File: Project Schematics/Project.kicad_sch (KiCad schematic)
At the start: 9 parts

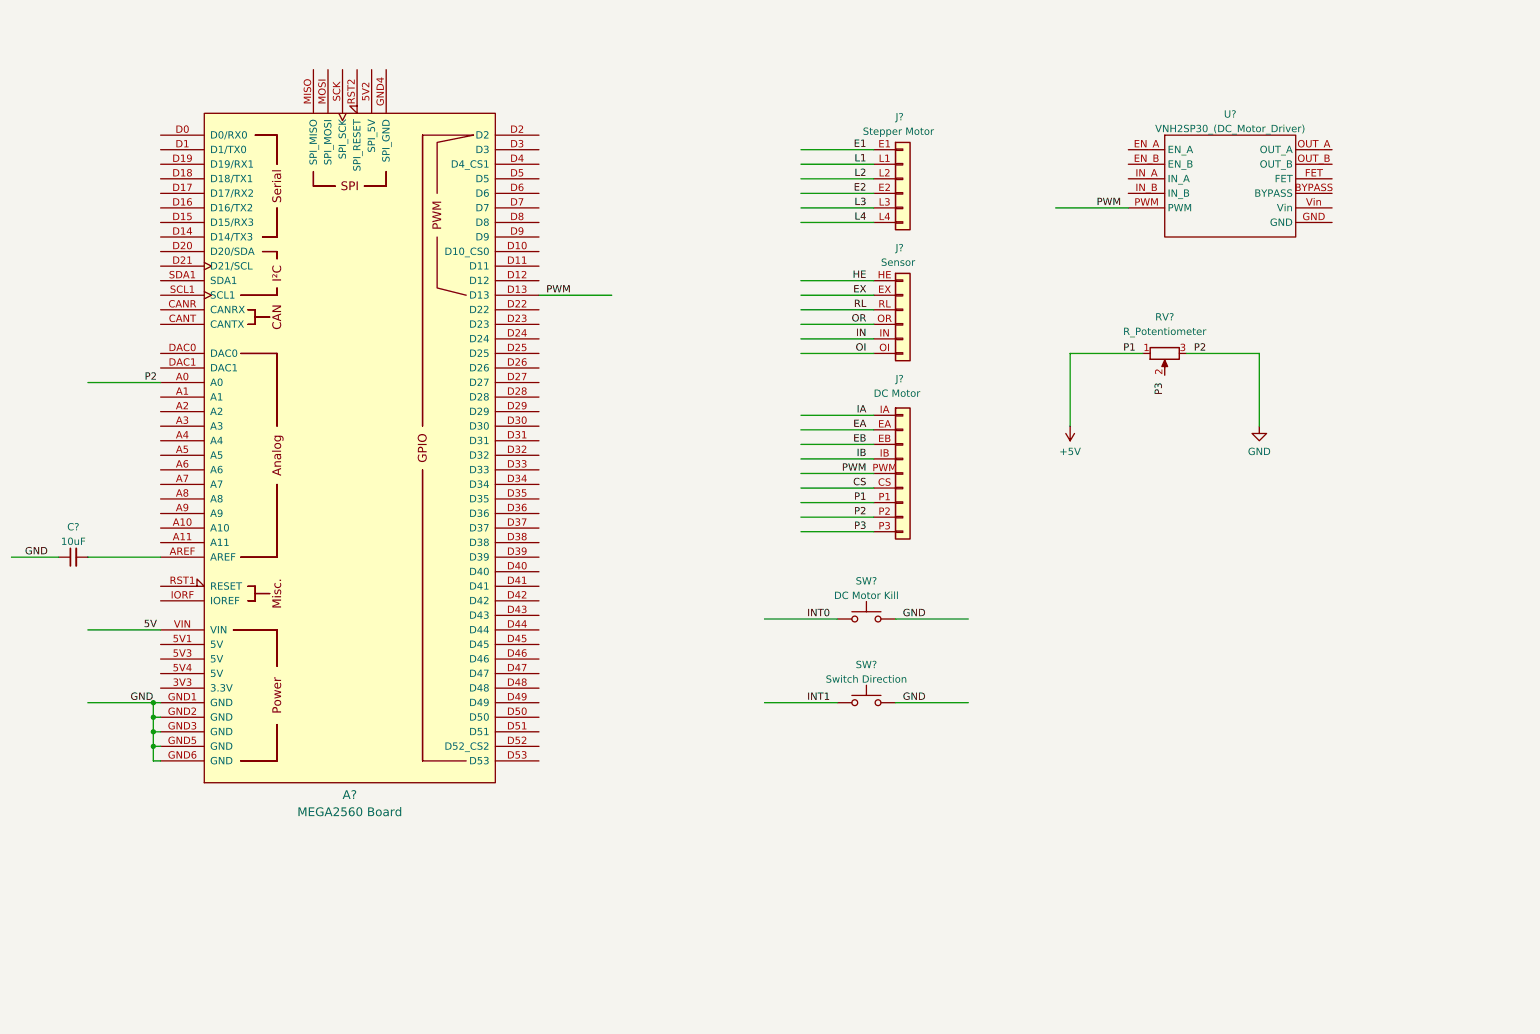
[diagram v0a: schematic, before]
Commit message: project schematic
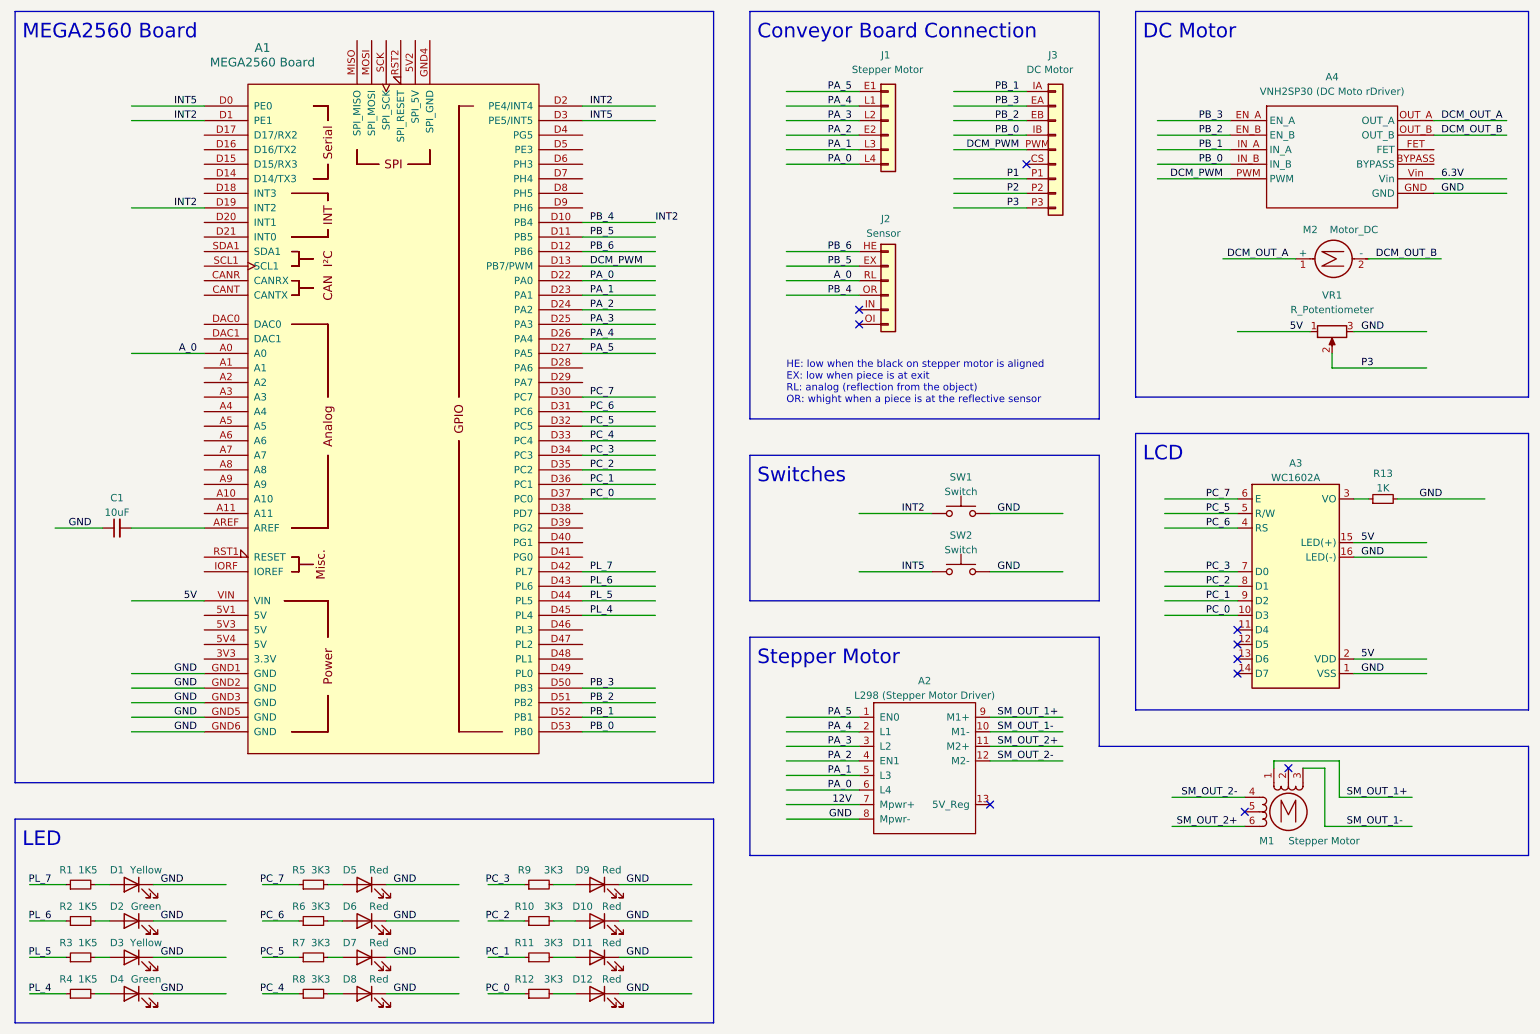
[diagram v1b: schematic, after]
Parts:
- added A2: L298 (Stepper Motor Driver), symbol Project:L298
- added A3: WC1602A, Display:WC1602A, symbol Project:LCD1602
- added D1, D3: Yellow, symbol Device:LED
- added D10, D11, D12, D5, D6, D7, D8, D9: Red, symbol Device:LED
- added D2, D4: Green, symbol Device:LED
- added M1: Stepper Motor, symbol Motor:Stepper_Motor_unipolar_6pin
- added M2: Motor_DC, symbol Motor:Motor_DC
- added R1, R2, R3, R4: 1K5, symbol Device:R_Small
- added R10, R11, R12, R5, R6, R7, R8, R9: 3K3, symbol Device:R_Small
- added R13: 1K, symbol Device:R_Small
- A4: renamed from U?; value VNH2SP30_(DC_Motor_Driver) -> VNH2SP30 (DC Moto rDriver)
- SW1: renamed from SW?; value DC Motor Kill -> Switch
- SW2: renamed from SW?; value Switch Direction -> Switch
- gave numbers to parts that had none: 6
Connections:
- net E1 is gone; now on net PA_5: J1.E1 (Pin_1)
- net E2 is gone; now on net PA_2: J1.E2 (Pin_4)
- net EA is gone; now on net PB_3: J3.EA (Pin_2)
- net EB is gone; now on net PB_2: J3.EB (Pin_3)
- net EX is gone; now on net PB_5: J2.EX (Pin_2)
- net HE is gone; now on net PB_6: J2.HE (Pin_1)
- net IA is gone; now on net PB_1: J3.IA (EA)
- net IB is gone; now on net PB_0: J3.IB (Pin_4)
- net INT0 is gone; now on net INT2: SW1.1
- net INT1 is gone; now on net INT5: SW2.1
- net L1 is gone; now on net PA_4: J1.L1 (Pin_2)
- net L2 is gone; now on net PA_3: J1.L2 (Pin_3)
- net L3 is gone; now on net PA_1: J1.L3 (Pin_5)
- net L4 is gone; now on net PA_0: J1.L4 (Pin_6)
- net OR is gone; now on net INT2: J2.OR (Pin_4)
- net 5V: now also VR1.1, A3.15 (LED(+)), A3.2 (VDD)
- net GND: now also A4.GND, A2.8 (Mpwr-), A3.1 (VSS), A3.16 (LED(-)), D1.1 (K), D10.1 (K), D11.1 (K), D12.1 (K), D2.1 (K), D3.1 (K), D4.1 (K), D5.1 (K), D6.1 (K), D7.1 (K), D8.1 (K), D9.1 (K), R13.2; no longer A1.A0, J3.P2 (Pin_8)
- net P3: now also VR1.2
- net INT5: now reaches A1.D0 (PE0)
- net INT5: now also A1.D3 (PE5/INT5)
- net INT2: now reaches A1.D1 (PE1)
- net INT2: now also A1.D10 (PB4), A1.D19 (INT2), A1.D2 (PE4/INT4)
- net PB_5: now reaches A1.D11 (PB5)
- net PB_6: now reaches A1.D12 (PB6)
- net PA_0: now reaches A1.D22 (PA0)
- net PA_0: now also A2.6 (L4)
- net PA_1: now reaches A1.D23 (PA1)
- net PA_1: now also A2.5 (L3)
- net PA_2: now reaches A1.D24 (PA2)
- net PA_2: now also A2.4 (EN1)
- net PA_3: now reaches A1.D25 (PA3)
- net PA_3: now also A2.3 (L2)
- net PA_4: now reaches A1.D26 (PA4)
- net PA_4: now also A2.2 (L1)
- net PA_5: now reaches A1.D27 (PA5)
- net PA_5: now also A2.1 (EN0)
- net PC_7: now reaches A1.D30 (PC7)
- net PC_7: now also A3.6 (E), R5.1
- net PC_6: now reaches A1.D31 (PC6)
- net PC_6: now also A3.4 (RS), R6.1
- net PC_5: now reaches A1.D32 (PC5)
- net PC_5: now also A3.5 (R/W), R7.1
- net PC_4: now reaches A1.D33 (PC4)
- net PC_4: now also R8.1
- net PC_3: now reaches A1.D34 (PC3)
- net PC_3: now also A3.7 (D0), R9.1
- net PC_2: now reaches A1.D35 (PC2)
- net PC_2: now also A3.8 (D1), R10.1
- net PC_1: now reaches A1.D36 (PC1)
- net PC_1: now also A3.9 (D2), R11.1
- net PC_0: now reaches A1.D37 (PC0)
- net PC_0: now also A3.10 (D3), R12.1
- net PL_7: now reaches A1.D42 (PL7)
- net PL_7: now also R1.1
- net PL_6: now reaches A1.D43 (PL6)
- net PL_6: now also R2.1
- net PL_5: now reaches A1.D44 (PL5)
- net PL_5: now also R3.1
- net PL_4: now reaches A1.D45 (PL4)
- net PL_4: now also R4.1
- net PB_3: now reaches A1.D50 (PB3)
- net PB_3: now also A4.EN_A
- net PB_2: now reaches A1.D51 (PB2)
- net PB_2: now also A4.EN_B
- net PB_1: now reaches A1.D52 (PB1)
- net PB_1: now also A4.IN_A
- net PB_0: now reaches A1.D53 (PB0)
- net PB_0: now also A4.IN_B
- net DCM_OUT_A: now reaches A4.OUT_A
- net DCM_OUT_A: now also M2.1 (+)
- net DCM_OUT_B: now reaches A4.OUT_B
- net DCM_OUT_B: now also M2.2 (-)
- net 6.3V: now reaches A4.Vin
- net +5V renamed P1
- net P1: no longer VR1.1
- net CS: no longer names the net of J3.CS (Pin_6)
- net IN: no longer names the net of J2.IN (Pin_5)
- net OI: no longer names the net of J2.OI (Pin_6)
- net PWM renamed DCM_PWM
- net RL renamed A_0
- net A_0: now also A1.A0
- new net: D1.2 (A), R1.2
- new net: D3.2 (A), R3.2
- new net: D12.2 (A), R12.2
- new net: D4.2 (A), R4.2
- new net: D6.2 (A), R6.2
- new net: D9.2 (A), R9.2
- new net: D10.2 (A), R10.2
- new net: D5.2 (A), R5.2
- new net: D2.2 (A), R2.2
- new net: D8.2 (A), R8.2
- new net: D7.2 (A), R7.2
- new net: A3.3 (VO), R13.1
- new net: D11.2 (A), R11.2
- new net 12V: A2.7 (Mpwr+)
- new net P2: J3.P2 (Pin_8)
- new net SM_OUT_1+: A2.9 (M1+), M1.1
- new net SM_OUT_1-: A2.10 (M1-), M1.3 (-)
- new net SM_OUT_2+: A2.11 (M2+), M1.6
- new net SM_OUT_2-: A2.12 (M2-), M1.4
- no-connect marks 0 -> 10
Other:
- note added: "Conveyor Board Connection"
- note added: "DC Motor"
- note added: "HE: low when the black on stepper motor is aligned EX: low when piece is at exit RL: analog (reflection from the object) OR: whight when a piece is at the reflective sensor"
- note added: "LCD"
- note added: "LED"
- note added: "MEGA2560 Board"
- note added: "Stepper Motor"
- note added: "Switches"
- title: (none) -> MECH 458/554 Project
- moved on the sheet: A4, C1, J1, J2, J3, SW1, SW2, VR1
